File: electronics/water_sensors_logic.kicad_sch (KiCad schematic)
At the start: 11 parts, among them J16 Conn_01x02, J20 water_sensor_conn, Q1 Q_PMOS_GDS, U16 ULN2003

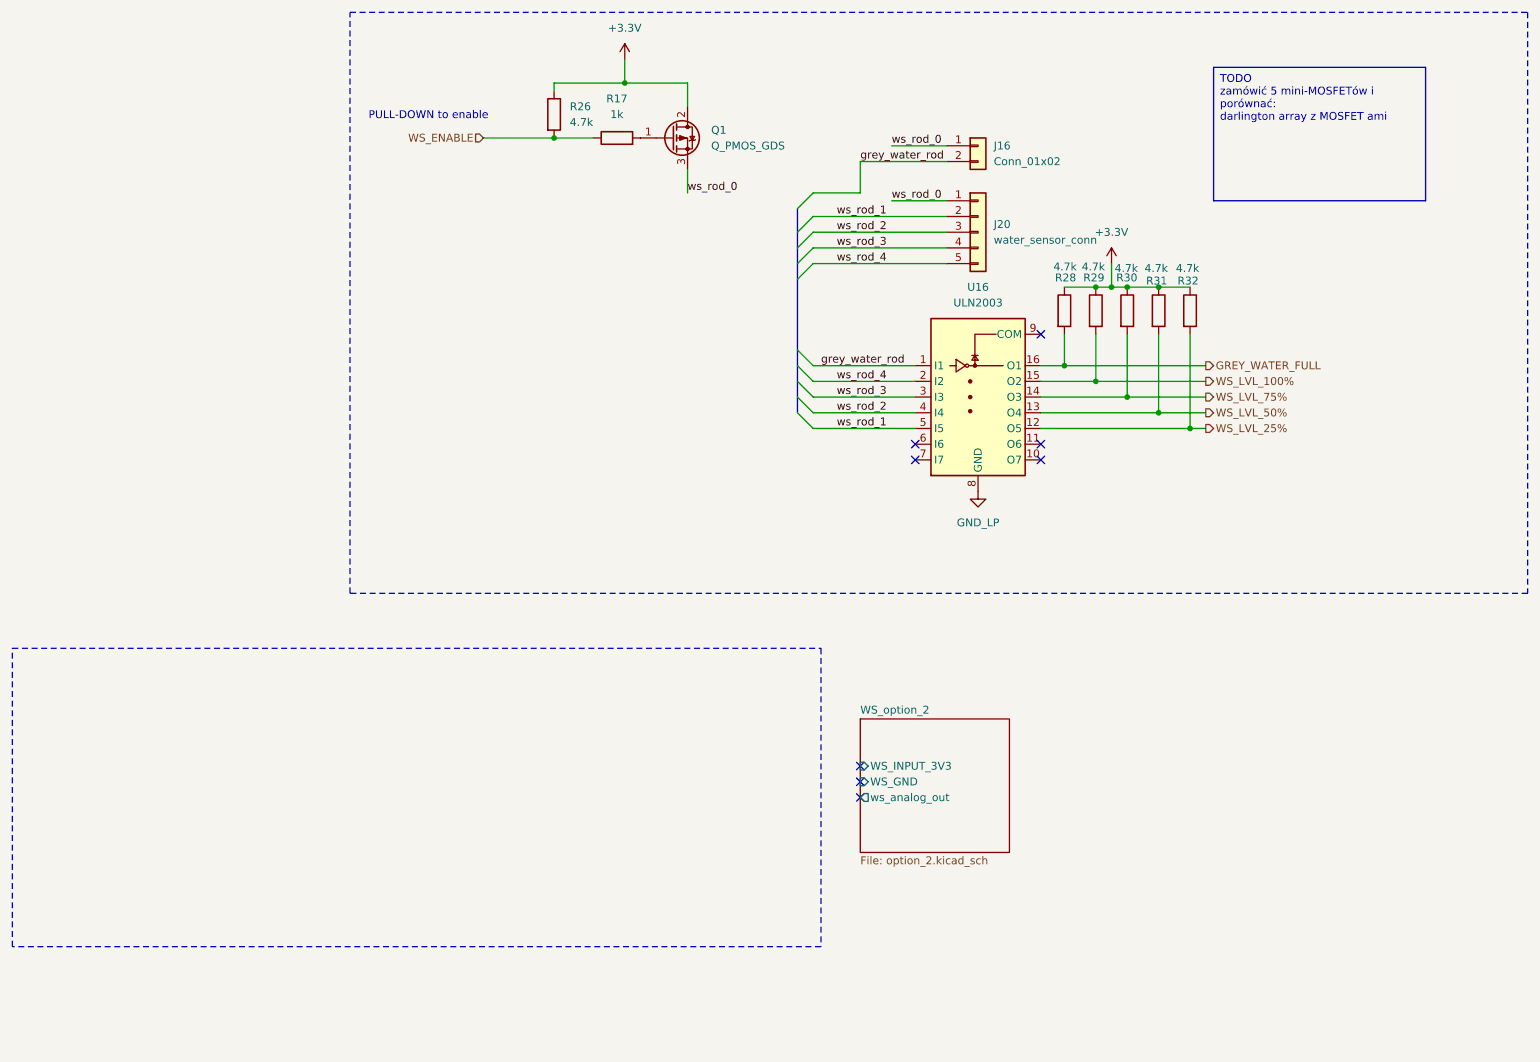
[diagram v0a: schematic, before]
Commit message: from dell
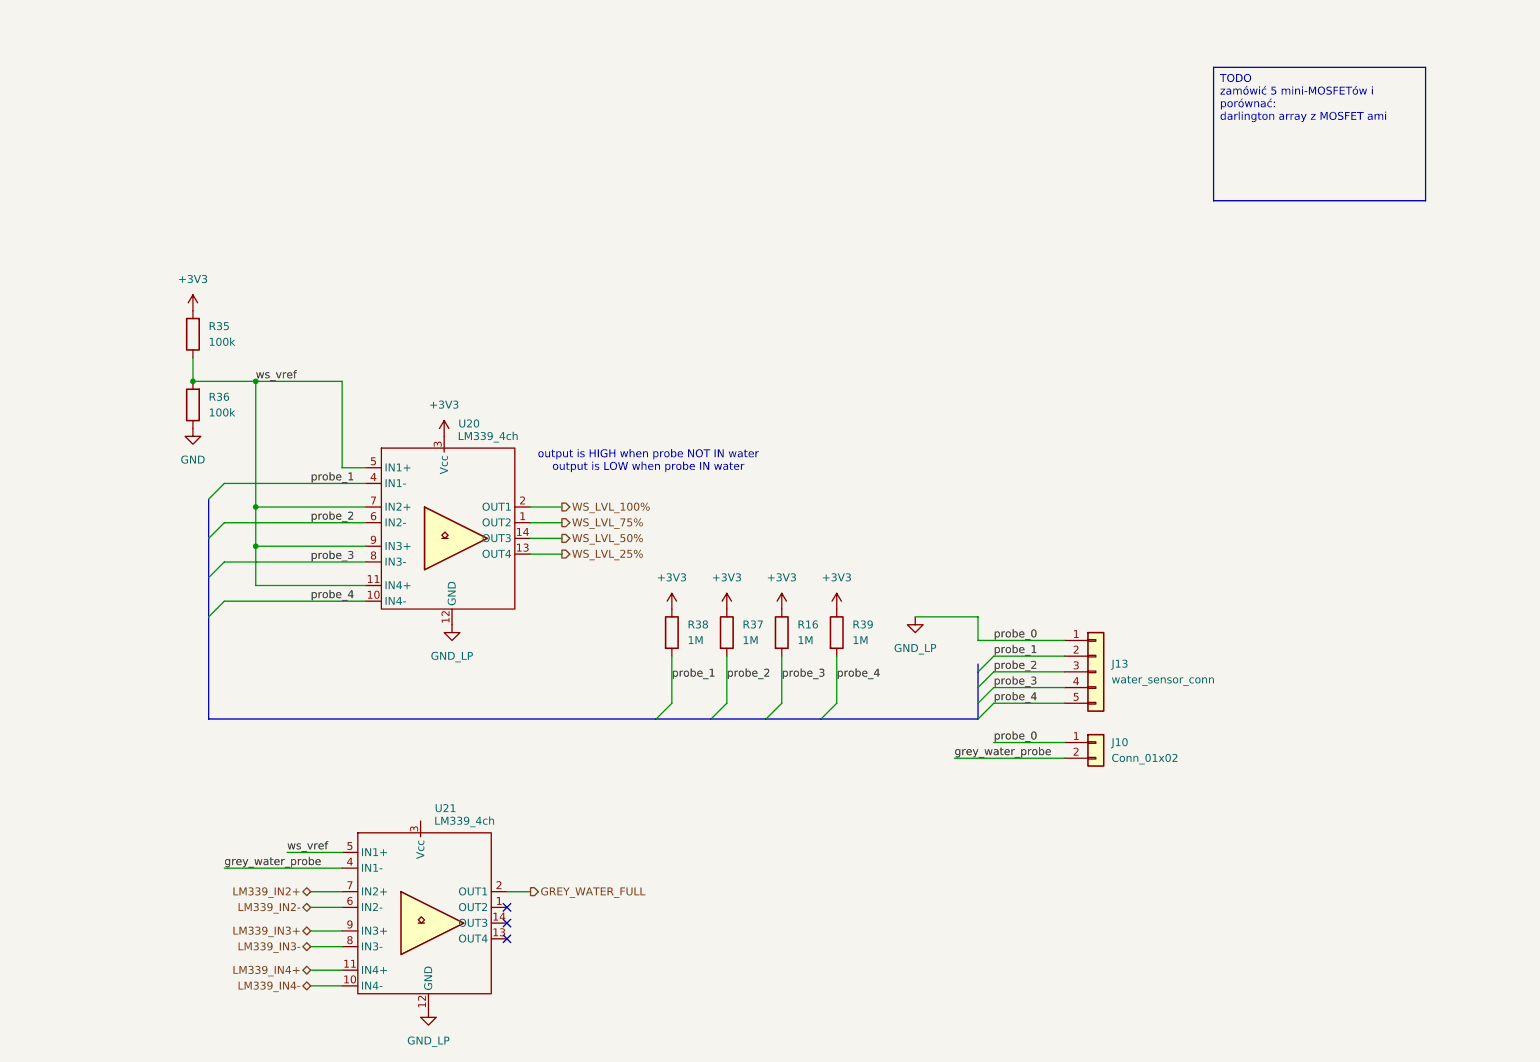
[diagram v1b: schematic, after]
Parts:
- removed J16: Conn_01x02, TerminalBlock:TerminalBlock_Xinya_XY308-2.54-2P_1x02_P2.54mm_Horizontal, symbol Connector_Generic:Conn_01x02
- removed J20: water_sensor_conn, TerminalBlock:TerminalBlock_Xinya_XY308-2.54-5P_1x05_P2.54mm_Horizontal, symbol Connector_Generic:Conn_01x05
- removed Q1: Q_PMOS_GDS, Package_TO_SOT_SMD:SOT-23_Handsoldering, symbol Device:Q_PMOS_GDS
- removed R17: 1k, Resistor_SMD:R_0805_2012Metric_Pad1.20x1.40mm_HandSolder, symbol Device:R
- removed R26, R28, R29, R30, R31, R32: 4.7k, Resistor_SMD:R_0805_2012Metric_Pad1.20x1.40mm_HandSolder, symbol Device:R
- removed U16: ULN2003, Package_SO:SO-16_3.9x9.9mm_P1.27mm, symbol Transistor_Array:ULN2003
- added J10: Conn_01x02, TerminalBlock:TerminalBlock_Xinya_XY308-2.54-2P_1x02_P2.54mm_Horizontal, symbol Connector_Generic:Conn_01x02
- added J13: water_sensor_conn, TerminalBlock:TerminalBlock_Xinya_XY308-2.54-5P_1x05_P2.54mm_Horizontal, symbol Connector_Generic:Conn_01x05
- added R16, R37, R38, R39: 1M, Resistor_SMD:R_0805_2012Metric_Pad1.20x1.40mm_HandSolder, symbol Device:R
- added R35, R36: 100k, Resistor_SMD:R_0805_2012Metric_Pad1.20x1.40mm_HandSolder, symbol Device:R
- added U20, U21: LM339_4ch, Package_SO:HTSSOP-14-1EP_4.4x5mm_P0.65mm_EP3.4x5mm_Mask3x3.1mm, symbol HeavyDuty:LM339_4ch
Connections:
- net GND_LP: now also J10.1 (Pin_1), J13.1 (Pin_1), U20.12 (GND), U21.12 (GND)
- net GREY_WATER_FULL: now also U21.2 (OUT1)
- net WS_LVL_100%: now also U20.2 (OUT1)
- net WS_LVL_25%: now also U20.13 (OUT4)
- net WS_LVL_50%: now also U20.14 (OUT3)
- net WS_LVL_75%: now also U20.1 (OUT2)
- new net +3V3: R16.1, R35.2, R37.1, R38.1, R39.1, U20.3 (Vcc)
- new net GND: R36.1
- new net LM339_IN2+: U21.7 (IN2+)
- new net LM339_IN2-: U21.6 (IN2-)
- new net LM339_IN3+: U21.9 (IN3+)
- new net LM339_IN3-: U21.8 (IN3-)
- new net LM339_IN4+: U21.11 (IN4+)
- new net LM339_IN4-: U21.10 (IN4-)
- new net grey_water_probe: J10.2 (Pin_2), U21.4 (IN1-)
- new net probe_1: J13.2 (Pin_2), R38.2, U20.4 (IN1-)
- new net probe_2: J13.3 (Pin_3), R37.2, U20.6 (IN2-)
- new net probe_3: J13.4 (Pin_4), R16.2, U20.8 (IN3-)
- new net probe_4: J13.5 (Pin_5), R39.2, U20.10 (IN4-)
- new net ws_vref: R35.1, R36.2, U20.11 (IN4+), U20.5 (IN1+), U20.7 (IN2+), U20.9 (IN3+), U21.5 (IN1+)
- no-connect marks 8 -> 3
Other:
- removed sheet WS_option_2
- note added: "output is HIGH when probe NOT IN water output is LOW when probe IN water"
- note removed: "PULL-DOWN to enable"
